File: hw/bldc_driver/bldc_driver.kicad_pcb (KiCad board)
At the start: 2 copper layers, 13 parts, among them Q1 Q_NMOS_DGS, U1 CH32V30xRxTx, U2 STGAP2SCM, U3 STGAP2SCM, U4 STGAP2SCM, U5 STGAP2SCM, U6 STGAP2SCM, U7 STGAP2SCM

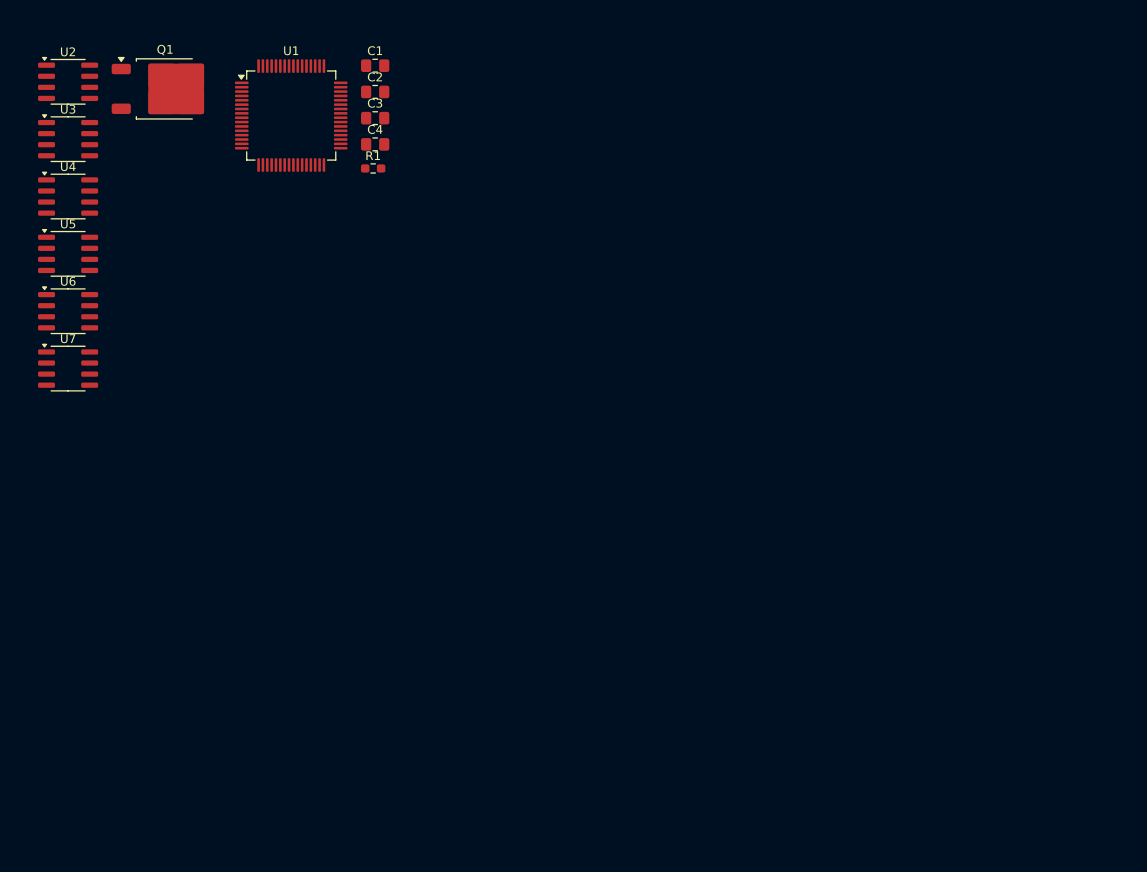
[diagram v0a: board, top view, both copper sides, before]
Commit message: feat: add CNCs
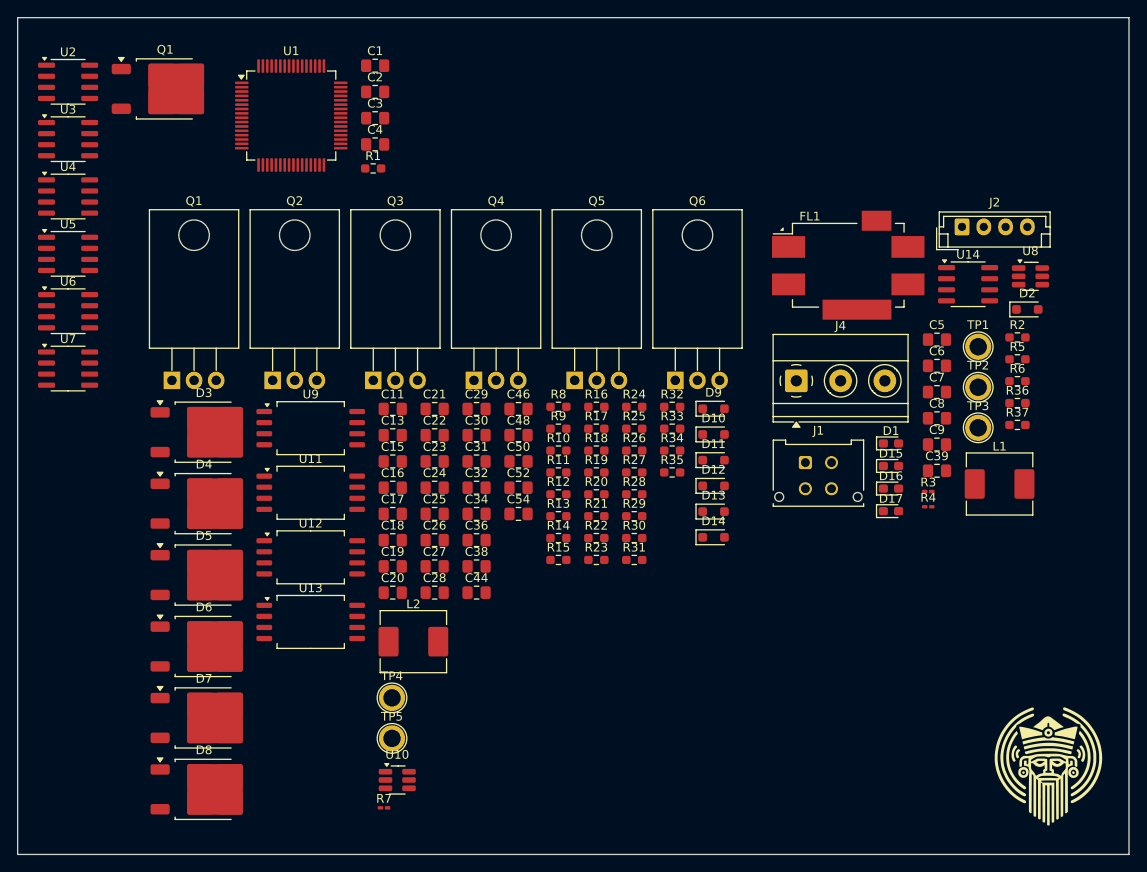
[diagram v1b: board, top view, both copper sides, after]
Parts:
- added C11: 0.1 µF, Capacitor_SMD:C_0805_2012Metric_Pad1.18x1.45mm_HandSolder, F.Cu at (114.5, 88.9)
- added C13: 0.1 µF, Capacitor_SMD:C_0805_2012Metric_Pad1.18x1.45mm_HandSolder, F.Cu at (114.5, 91.9)
- added C15: 0.1 µF, Capacitor_SMD:C_0805_2012Metric_Pad1.18x1.45mm_HandSolder, F.Cu at (114.5, 94.9)
- added C16: 10 µF, Capacitor_SMD:C_0805_2012Metric_Pad1.18x1.45mm_HandSolder, F.Cu at (114.5, 97.9)
- added C17: 0.1 µF, Capacitor_SMD:C_0805_2012Metric_Pad1.18x1.45mm_HandSolder, F.Cu at (114.5, 100.9)
- added C18: 0.1 µF, Capacitor_SMD:C_0805_2012Metric_Pad1.18x1.45mm_HandSolder, F.Cu at (114.5, 103.9)
- added C19: 22 µF, Capacitor_SMD:C_0805_2012Metric_Pad1.18x1.45mm_HandSolder, F.Cu at (114.5, 107.0)
- added C20: 22 µF, Capacitor_SMD:C_0805_2012Metric_Pad1.18x1.45mm_HandSolder, F.Cu at (114.5, 110.0)
- added C21: 0.1 µF, Capacitor_SMD:C_0805_2012Metric_Pad1.18x1.45mm_HandSolder, F.Cu at (119.3, 88.9)
- added C22: 0.1 µF, Capacitor_SMD:C_0805_2012Metric_Pad1.18x1.45mm_HandSolder, F.Cu at (119.3, 91.9)
- added C23: 330 pF, Capacitor_SMD:C_0805_2012Metric_Pad1.18x1.45mm_HandSolder, F.Cu at (119.3, 94.9)
- added C24: 330 pF, Capacitor_SMD:C_0805_2012Metric_Pad1.18x1.45mm_HandSolder, F.Cu at (119.3, 97.9)
- added C25: 0.1 µF, Capacitor_SMD:C_0805_2012Metric_Pad1.18x1.45mm_HandSolder, F.Cu at (119.3, 100.9)
- added C26: 0.1 µF, Capacitor_SMD:C_0805_2012Metric_Pad1.18x1.45mm_HandSolder, F.Cu at (119.3, 103.9)
- added C27: 330 pF, Capacitor_SMD:C_0805_2012Metric_Pad1.18x1.45mm_HandSolder, F.Cu at (119.3, 107.0)
- added C28: 0.1 µF, Capacitor_SMD:C_0805_2012Metric_Pad1.18x1.45mm_HandSolder, F.Cu at (119.3, 110.0)
- added C29: 0.1 µF, Capacitor_SMD:C_0805_2012Metric_Pad1.18x1.45mm_HandSolder, F.Cu at (124.2, 88.9)
- added C30: 330 pF, Capacitor_SMD:C_0805_2012Metric_Pad1.18x1.45mm_HandSolder, F.Cu at (124.2, 91.9)
- added C31: 0.1 µF, Capacitor_SMD:C_0805_2012Metric_Pad1.18x1.45mm_HandSolder, F.Cu at (124.2, 94.9)
- added C32: 0.1 µF, Capacitor_SMD:C_0805_2012Metric_Pad1.18x1.45mm_HandSolder, F.Cu at (124.2, 97.9)
- added C34: 0.1 µF, Capacitor_SMD:C_0805_2012Metric_Pad1.18x1.45mm_HandSolder, F.Cu at (124.2, 100.9)
- added C36: 0.1 µF, Capacitor_SMD:C_0805_2012Metric_Pad1.18x1.45mm_HandSolder, F.Cu at (124.2, 103.9)
- added C38: 0.1 µF, Capacitor_SMD:C_0805_2012Metric_Pad1.18x1.45mm_HandSolder, F.Cu at (124.2, 107.0)
- added C39: 0.1 µF, Capacitor_SMD:C_0805_2012Metric_Pad1.18x1.45mm_HandSolder, F.Cu at (177.0, 96.0)
- added C44: 0.1 µF, Capacitor_SMD:C_0805_2012Metric_Pad1.18x1.45mm_HandSolder, F.Cu at (124.2, 110.0)
- added C46: 0.1 µF, Capacitor_SMD:C_0805_2012Metric_Pad1.18x1.45mm_HandSolder, F.Cu at (129.0, 88.9)
- added C48: 0.1 µF, Capacitor_SMD:C_0805_2012Metric_Pad1.18x1.45mm_HandSolder, F.Cu at (129.0, 91.9)
- added C5: 10 µF, Capacitor_SMD:C_0805_2012Metric_Pad1.18x1.45mm_HandSolder, F.Cu at (177.0, 80.9)
- added C50: 0.1 µF, Capacitor_SMD:C_0805_2012Metric_Pad1.18x1.45mm_HandSolder, F.Cu at (129.0, 94.9)
- added C52: 0.1 µF, Capacitor_SMD:C_0805_2012Metric_Pad1.18x1.45mm_HandSolder, F.Cu at (129.0, 97.9)
- added C54: 0.1 µF, Capacitor_SMD:C_0805_2012Metric_Pad1.18x1.45mm_HandSolder, F.Cu at (129.0, 100.9)
- added C6: 0.1 µF, Capacitor_SMD:C_0805_2012Metric_Pad1.18x1.45mm_HandSolder, F.Cu at (177.0, 83.9)
- added C7: 0.1 µF, Capacitor_SMD:C_0805_2012Metric_Pad1.18x1.45mm_HandSolder, F.Cu at (177.0, 87.0)
- added C8: 22 µF, Capacitor_SMD:C_0805_2012Metric_Pad1.18x1.45mm_HandSolder, F.Cu at (177.0, 90.0)
- added C9: 22 µF, Capacitor_SMD:C_0805_2012Metric_Pad1.18x1.45mm_HandSolder, F.Cu at (177.0, 93.0)
- added D1: KT-0603W, LED_SMD:LED_0603_1608Metric_Pad1.05x0.95mm_HandSolder, F.Cu at (171.7, 92.8)
- added D10: 1N4148WS, Diode_SMD:D_SOD-323_HandSoldering, F.Cu at (151.3, 91.8)
- added D11: 1N4148WS, Diode_SMD:D_SOD-323_HandSoldering, F.Cu at (151.3, 94.8)
- added D12: 1N4148WS, Diode_SMD:D_SOD-323_HandSoldering, F.Cu at (151.3, 97.7)
- added D13: 1N4148WS, Diode_SMD:D_SOD-323_HandSoldering, F.Cu at (151.3, 100.7)
- added D14: 1N4148WS, Diode_SMD:D_SOD-323_HandSoldering, F.Cu at (151.3, 103.6)
- added D15: KT-0603W, LED_SMD:LED_0603_1608Metric_Pad1.05x0.95mm_HandSolder, F.Cu at (171.7, 95.4)
- added D16: KT-0603W, LED_SMD:LED_0603_1608Metric_Pad1.05x0.95mm_HandSolder, F.Cu at (171.7, 98.0)
- added D17: KT-0603W, LED_SMD:LED_0603_1608Metric_Pad1.05x0.95mm_HandSolder, F.Cu at (171.7, 100.6)
- added D2: PESD15VL1BA, Diode_SMD:D_SOD-323_HandSoldering, F.Cu at (187.3, 77.5)
- added D3: MBR20100DT, Package_TO_SOT_SMD:TO-252-2, F.Cu at (92.9, 91.6)
- added D4: MBR20100DT, Package_TO_SOT_SMD:TO-252-2, F.Cu at (92.9, 99.8)
- added D5: MBR20100DT, Package_TO_SOT_SMD:TO-252-2, F.Cu at (92.9, 108.0)
- added D6: MBR20100DT, Package_TO_SOT_SMD:TO-252-2, F.Cu at (92.9, 116.1)
- added D7: MBR20100DT, Package_TO_SOT_SMD:TO-252-2, F.Cu at (92.9, 124.3)
- added D8: MBR20100DT, Package_TO_SOT_SMD:TO-252-2, F.Cu at (92.9, 132.5)
- added D9: 1N4148WS, Diode_SMD:D_SOD-323_HandSoldering, F.Cu at (151.3, 88.9)
- added FL1: BNX025, Filter:Filter_Murata_BNX025, F.Cu at (166.8, 72.4)
- added J1: 430450412, Connector_Molex:Molex_Micro-Fit_3.0_43045-0412_2x02_P3.00mm_Vertical, F.Cu at (161.9, 95.0)
- added J2: B4B-EH-A(LF)(SN), Connector_JST:JST_EH_B4B-EH-A_1x04_P2.50mm_Vertical, F.Cu at (179.8, 68.0)
- added J4: 1733583, TerminalBlock_Phoenix:TerminalBlock_Phoenix_MKDS-1,5-3-5.08_1x03_P5.08mm_Horizontal, F.Cu at (160.8, 85.7)
- added L1: KOHER_MDA7030 15uH, Inductor_SMD:L_KOHERelec_MDA7030, F.Cu at (184.2, 97.5)
- added L2: KOHER_MDA7030 15uH, Inductor_SMD:L_KOHERelec_MDA7030, F.Cu at (116.9, 115.6)
- added Q1: IRF540N, Package_TO_SOT_THT:TO-220-3_Horizontal_TabDown, F.Cu at (89.2, 85.6)
- added Q2: IRF540N, Package_TO_SOT_THT:TO-220-3_Horizontal_TabDown, F.Cu at (100.8, 85.6)
- added Q3: IRF540N, Package_TO_SOT_THT:TO-220-3_Horizontal_TabDown, F.Cu at (112.3, 85.6)
- added Q4: IRF540N, Package_TO_SOT_THT:TO-220-3_Horizontal_TabDown, F.Cu at (123.8, 85.6)
- added Q5: IRF540N, Package_TO_SOT_THT:TO-220-3_Horizontal_TabDown, F.Cu at (135.4, 85.6)
- added Q6: IRF540N, Package_TO_SOT_THT:TO-220-3_Horizontal_TabDown, F.Cu at (146.9, 85.6)
- added R10: 12 ohm, Resistor_SMD:R_0603_1608Metric_Pad0.98x0.95mm_HandSolder, F.Cu at (133.5, 93.7)
- added R11: 12 ohm, Resistor_SMD:R_0603_1608Metric_Pad0.98x0.95mm_HandSolder, F.Cu at (133.5, 96.2)
- added R12: 12 ohm, Resistor_SMD:R_0603_1608Metric_Pad0.98x0.95mm_HandSolder, F.Cu at (133.5, 98.7)
- added R13: 12 ohm, Resistor_SMD:R_0603_1608Metric_Pad0.98x0.95mm_HandSolder, F.Cu at (133.5, 101.2)
- added R14: 12 ohm, Resistor_SMD:R_0603_1608Metric_Pad0.98x0.95mm_HandSolder, F.Cu at (133.5, 103.7)
- added R15: 12 ohm, Resistor_SMD:R_0603_1608Metric_Pad0.98x0.95mm_HandSolder, F.Cu at (133.5, 106.2)
- added R16: 12 ohm, Resistor_SMD:R_0603_1608Metric_Pad0.98x0.95mm_HandSolder, F.Cu at (137.9, 88.6)
- added R17: 12 ohm, Resistor_SMD:R_0603_1608Metric_Pad0.98x0.95mm_HandSolder, F.Cu at (137.9, 91.2)
- added R18: 470 kohm, Resistor_SMD:R_0603_1608Metric_Pad0.98x0.95mm_HandSolder, F.Cu at (137.9, 93.7)
- added R19: 10 kohm, Resistor_SMD:R_0603_1608Metric_Pad0.98x0.95mm_HandSolder, F.Cu at (137.9, 96.2)
- added R2: 100 Ohm, Resistor_SMD:R_0603_1608Metric_Pad0.98x0.95mm_HandSolder, F.Cu at (186.2, 80.7)
- added R20: 470 kohm, Resistor_SMD:R_0603_1608Metric_Pad0.98x0.95mm_HandSolder, F.Cu at (137.9, 98.7)
- added R21: 10 kohm, Resistor_SMD:R_0603_1608Metric_Pad0.98x0.95mm_HandSolder, F.Cu at (137.9, 101.2)
- added R22: 470 kohm, Resistor_SMD:R_0603_1608Metric_Pad0.98x0.95mm_HandSolder, F.Cu at (137.9, 103.7)
- added R23: 10 kohm, Resistor_SMD:R_0603_1608Metric_Pad0.98x0.95mm_HandSolder, F.Cu at (137.9, 106.2)
- added R24: 12 ohm, Resistor_SMD:R_0603_1608Metric_Pad0.98x0.95mm_HandSolder, F.Cu at (142.2, 88.6)
- added R25: 12 ohm, Resistor_SMD:R_0603_1608Metric_Pad0.98x0.95mm_HandSolder, F.Cu at (142.2, 91.2)
- added R26: 12 ohm, Resistor_SMD:R_0603_1608Metric_Pad0.98x0.95mm_HandSolder, F.Cu at (142.2, 93.7)
- added R27: 12 ohm, Resistor_SMD:R_0603_1608Metric_Pad0.98x0.95mm_HandSolder, F.Cu at (142.2, 96.2)
- added R28: 12 ohm, Resistor_SMD:R_0603_1608Metric_Pad0.98x0.95mm_HandSolder, F.Cu at (142.2, 98.7)
- added R29: 12 ohm, Resistor_SMD:R_0603_1608Metric_Pad0.98x0.95mm_HandSolder, F.Cu at (142.2, 101.2)
- added R3: 0 ohm, Resistor_SMD:R_0201_0603Metric_Pad0.64x0.40mm_HandSolder, F.Cu at (176.0, 98.4)
- added R30: 12 ohm, Resistor_SMD:R_0603_1608Metric_Pad0.98x0.95mm_HandSolder, F.Cu at (142.2, 103.7)
- added R31: 12 ohm, Resistor_SMD:R_0603_1608Metric_Pad0.98x0.95mm_HandSolder, F.Cu at (142.2, 106.2)
- added R32: 12 ohm, Resistor_SMD:R_0603_1608Metric_Pad0.98x0.95mm_HandSolder, F.Cu at (146.6, 88.6)
- added R33: 12 ohm, Resistor_SMD:R_0603_1608Metric_Pad0.98x0.95mm_HandSolder, F.Cu at (146.6, 91.2)
- added R34: 12 ohm, Resistor_SMD:R_0603_1608Metric_Pad0.98x0.95mm_HandSolder, F.Cu at (146.6, 93.7)
- added R35: 12 ohm, Resistor_SMD:R_0603_1608Metric_Pad0.98x0.95mm_HandSolder, F.Cu at (146.6, 96.2)
- added R36: 100 Ohm, Resistor_SMD:R_0603_1608Metric_Pad0.98x0.95mm_HandSolder, F.Cu at (186.2, 88.2)
- added R37: 100 Ohm, Resistor_SMD:R_0603_1608Metric_Pad0.98x0.95mm_HandSolder, F.Cu at (186.2, 90.7)
- added R4: 100 kohm, Resistor_SMD:R_0201_0603Metric_Pad0.64x0.40mm_HandSolder, F.Cu at (176.0, 100.1)
- added R5: 22 kohm, Resistor_SMD:R_0603_1608Metric_Pad0.98x0.95mm_HandSolder, F.Cu at (186.2, 83.2)
- added R6: 100 Ohm, Resistor_SMD:R_0603_1608Metric_Pad0.98x0.95mm_HandSolder, F.Cu at (186.2, 85.7)
- added R7: 0 ohm, Resistor_SMD:R_0201_0603Metric_Pad0.64x0.40mm_HandSolder, F.Cu at (113.5, 134.7)
- added R8: 200 kohm, Resistor_SMD:R_0603_1608Metric_Pad0.98x0.95mm_HandSolder, F.Cu at (133.5, 88.6)
- added R9: 27 kohm, Resistor_SMD:R_0603_1608Metric_Pad0.98x0.95mm_HandSolder, F.Cu at (133.5, 91.2)
- added TP1: TestPoint_Flag, TestPoint:TestPoint_Plated_Hole_D2.0mm, F.Cu at (181.7, 81.8)
- added TP2: TestPoint_Flag, TestPoint:TestPoint_Plated_Hole_D2.0mm, F.Cu at (181.7, 86.4)
- added TP3: TestPoint_Flag, TestPoint:TestPoint_Plated_Hole_D2.0mm, F.Cu at (181.7, 91.1)
- added TP4: TestPoint_Flag, TestPoint:TestPoint_Plated_Hole_D2.0mm, F.Cu at (114.5, 122.0)
- added TP5: TestPoint_Flag, TestPoint:TestPoint_Plated_Hole_D2.0mm, F.Cu at (114.5, 126.7)
- added U10: TPS54202DDC, Package_TO_SOT_SMD:SOT-23-6_Handsoldering, F.Cu at (115.0, 131.5)
- added U11: AMC1200BDWV, Package_SO:SOIC-8_7.5x5.85mm_P1.27mm, F.Cu at (105.1, 98.5)
- added U12: AMC1200BDWV, Package_SO:SOIC-8_7.5x5.85mm_P1.27mm, F.Cu at (105.1, 105.9)
- added U13: AMC1200BDWV, Package_SO:SOIC-8_7.5x5.85mm_P1.27mm, F.Cu at (105.1, 113.3)
- added U14: SN65HVD230, Package_SO:SOIC-8_3.9x4.9mm_P1.27mm, F.Cu at (180.5, 74.6)
- added U8: TPS54202DDC, Package_TO_SOT_SMD:SOT-23-6_Handsoldering, F.Cu at (187.7, 73.7)
- added U9: AMC1200BDWV, Package_SO:SOIC-8_7.5x5.85mm_P1.27mm, F.Cu at (105.1, 91.1)
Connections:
- U1 pad 10: /Motor/PH_V_HI -> /Motor/W_ADC_P
- U1 pad 11: /Motor/PH_V_LO -> /Motor/SHUNT_CURR_P
- U1 pad 24: /Motor/PH_W_HI -> unconnected-(U1-PC4-Pad24)
- U1 pad 25: /Motor/PH_W_LO -> unconnected-(U1-PC5-Pad25)
- U1 pad 34: unconnected-(U1-PB13-Pad34) -> Net-(D15-A)
- U1 pad 35: unconnected-(U1-PB14-Pad35) -> Net-(D16-A)
- U1 pad 36: unconnected-(U1-PB15-Pad36) -> Net-(D17-A)
- U1 pad 37: unconnected-(U1-PC6-Pad37) -> /Motor/PH_U_HI
- U1 pad 38: unconnected-(U1-PC7-Pad38) -> /Motor/PH_U_LO
- U1 pad 39: unconnected-(U1-PC8-Pad39) -> /Motor/PH_V_HI
- U1 pad 40: unconnected-(U1-PC9-Pad40) -> /Motor/PH_V_LO
- U1 pad 44: unconnected-(U1-PA11-Pad44) -> /CAN_RX
- U1 pad 45: unconnected-(U1-PA12-Pad45) -> /CAN_TX
- U1 pad 46: unconnected-(U1-SWDIO-Pad46) -> Net-(J2-Pin_3)
- U1 pad 49: unconnected-(U1-SWCLK-Pad49) -> Net-(J2-Pin_2)
- U1 pad 51: unconnected-(U1-PC10-Pad51) -> /Motor/PH_W_HI
- U1 pad 52: unconnected-(U1-PC11-Pad52) -> /Motor/PH_W_LO
- U1 pad 8: /Motor/PH_U_HI -> /Motor/U_ADC_P
- U1 pad 9: /Motor/PH_U_LO -> /Motor/V_ADC_P
- U2 pad 1: unconnected-(U2-VDD-Pad1) -> +3V3
- U2 pad 4: unconnected-(U2-GND-Pad4) -> GND
- U2 pad 5: unconnected-(U2-VH-Pad5) -> +VDC
- U2 pad 6: unconnected-(U2-GOUT-Pad6) -> Net-(D9-K)
- U2 pad 7: unconnected-(U2-CLAMP-Pad7) -> Net-(Q2-G)
- U2 pad 8: unconnected-(U2-GNDISO-Pad8) -> GNDPWR
- U3 pad 1: unconnected-(U3-VDD-Pad1) -> +3V3
- U3 pad 4: unconnected-(U3-GND-Pad4) -> GND
- U3 pad 5: unconnected-(U3-VH-Pad5) -> +VDC
- U3 pad 6: unconnected-(U3-GOUT-Pad6) -> Net-(D10-K)
- U3 pad 7: unconnected-(U3-CLAMP-Pad7) -> Net-(Q1-G)
- U3 pad 8: unconnected-(U3-GNDISO-Pad8) -> GNDPWR
- U4 pad 1: unconnected-(U4-VDD-Pad1) -> +3V3
- U4 pad 4: unconnected-(U4-GND-Pad4) -> GND
- U4 pad 5: unconnected-(U4-VH-Pad5) -> +VDC
- U4 pad 6: unconnected-(U4-GOUT-Pad6) -> Net-(D11-K)
- U4 pad 7: unconnected-(U4-CLAMP-Pad7) -> Net-(Q3-G)
- U4 pad 8: unconnected-(U4-GNDISO-Pad8) -> GNDPWR
- U5 pad 1: unconnected-(U5-VDD-Pad1) -> +3V3
- U5 pad 4: unconnected-(U5-GND-Pad4) -> GND
- U5 pad 5: unconnected-(U5-VH-Pad5) -> +VDC
- U5 pad 6: unconnected-(U5-GOUT-Pad6) -> Net-(D12-K)
- U5 pad 7: unconnected-(U5-CLAMP-Pad7) -> Net-(Q4-G)
- U5 pad 8: unconnected-(U5-GNDISO-Pad8) -> GNDPWR
- U6 pad 1: unconnected-(U6-VDD-Pad1) -> +3V3
- U6 pad 4: unconnected-(U6-GND-Pad4) -> GND
- U6 pad 5: unconnected-(U6-VH-Pad5) -> +VDC
- U6 pad 6: unconnected-(U6-GOUT-Pad6) -> Net-(D13-K)
- U6 pad 7: unconnected-(U6-CLAMP-Pad7) -> Net-(Q5-G)
- U6 pad 8: unconnected-(U6-GNDISO-Pad8) -> GNDPWR
- U7 pad 1: unconnected-(U7-VDD-Pad1) -> +3V3
- U7 pad 4: unconnected-(U7-GND-Pad4) -> GND
- U7 pad 5: unconnected-(U7-VH-Pad5) -> +VDC
- U7 pad 6: unconnected-(U7-GOUT-Pad6) -> Net-(D14-K)
- U7 pad 7: unconnected-(U7-CLAMP-Pad7) -> Net-(Q6-G)
- U7 pad 8: unconnected-(U7-GNDISO-Pad8) -> GNDPWR
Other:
- board outline added: 127.5 x 96 mm
